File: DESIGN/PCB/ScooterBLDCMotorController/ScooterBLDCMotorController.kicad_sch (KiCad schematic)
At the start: 34 parts, among them J1 M1 OUTPUT, J10 RC_ENABLE, J11 TO M2 ENCODER, J12 M2 INPUT, J13 Conn_01x01_Male, J14 Conn_01x01_Male, J2 TO M1 ENCODER, J3 M1 INPUT, J4 M2 OUTPUT, J5 I2C, J6 TEST SWITCH, J7 RC CH 1, J8 RC CH 2, J9 RC_PWR, U1 , U10 , U2 SN74HC14NR, U3 , U4 Teensy4.0, U5 SN74HC14NR, U6 , U7 , U8 5V_StepUpDown_Voltage_Regulat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, U9 3V_StepUpDown_Voltage_Regulat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

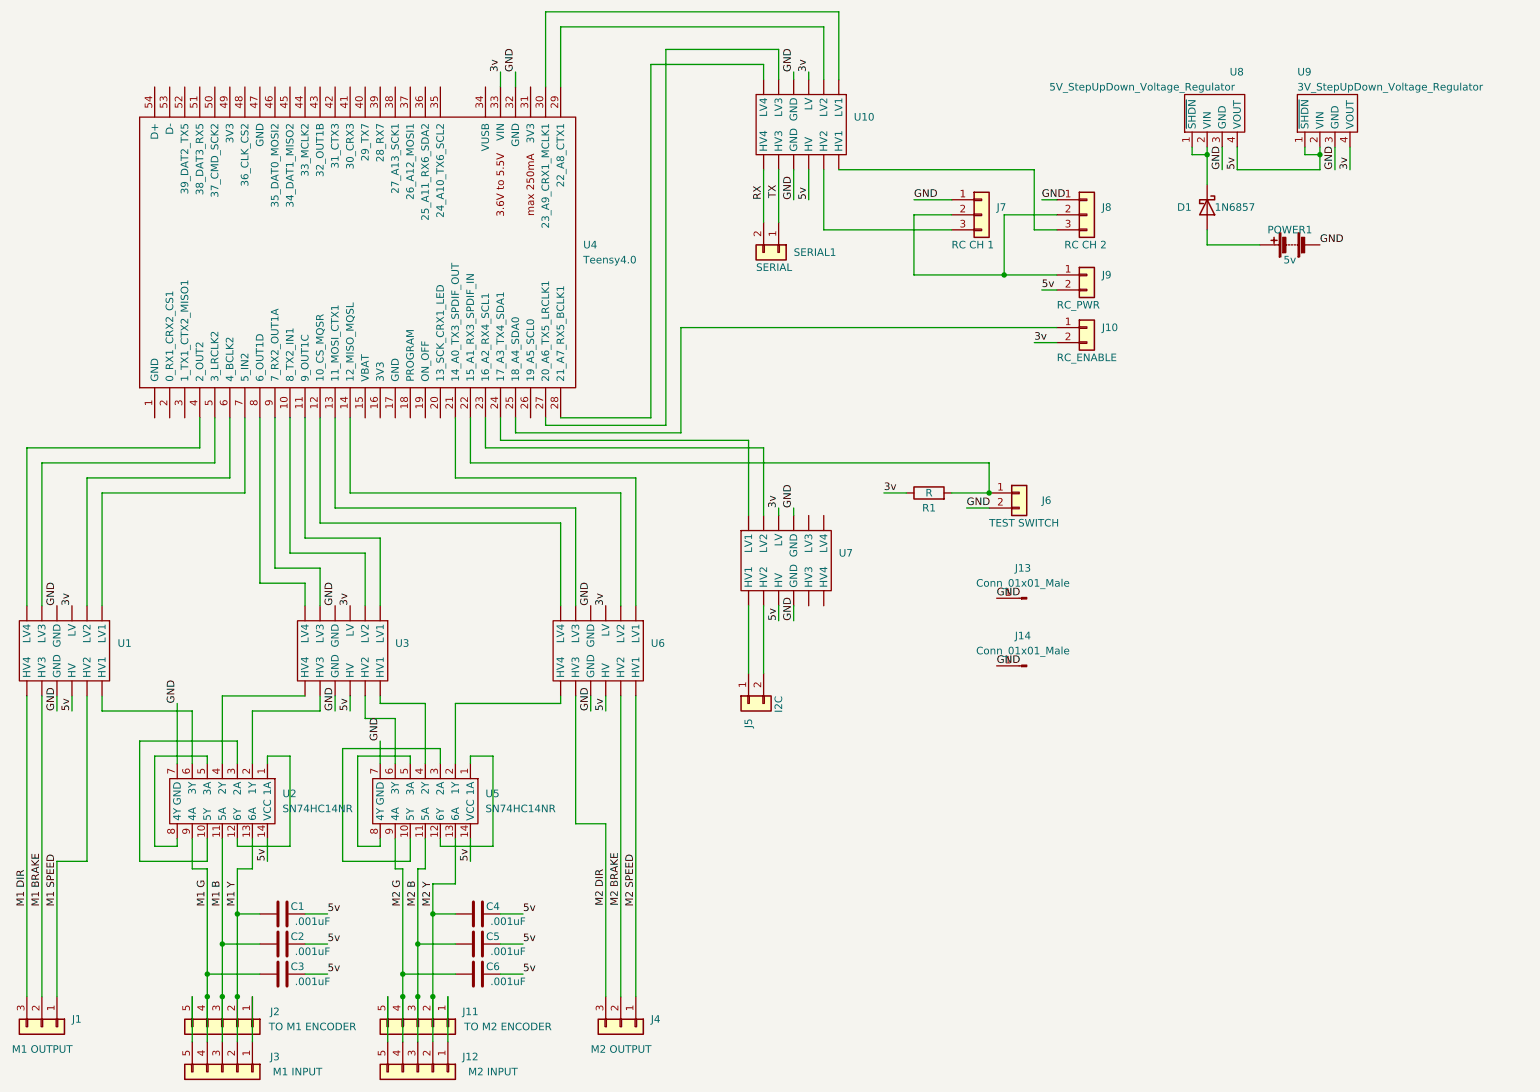
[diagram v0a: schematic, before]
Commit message: Revision 1.3 for PCB
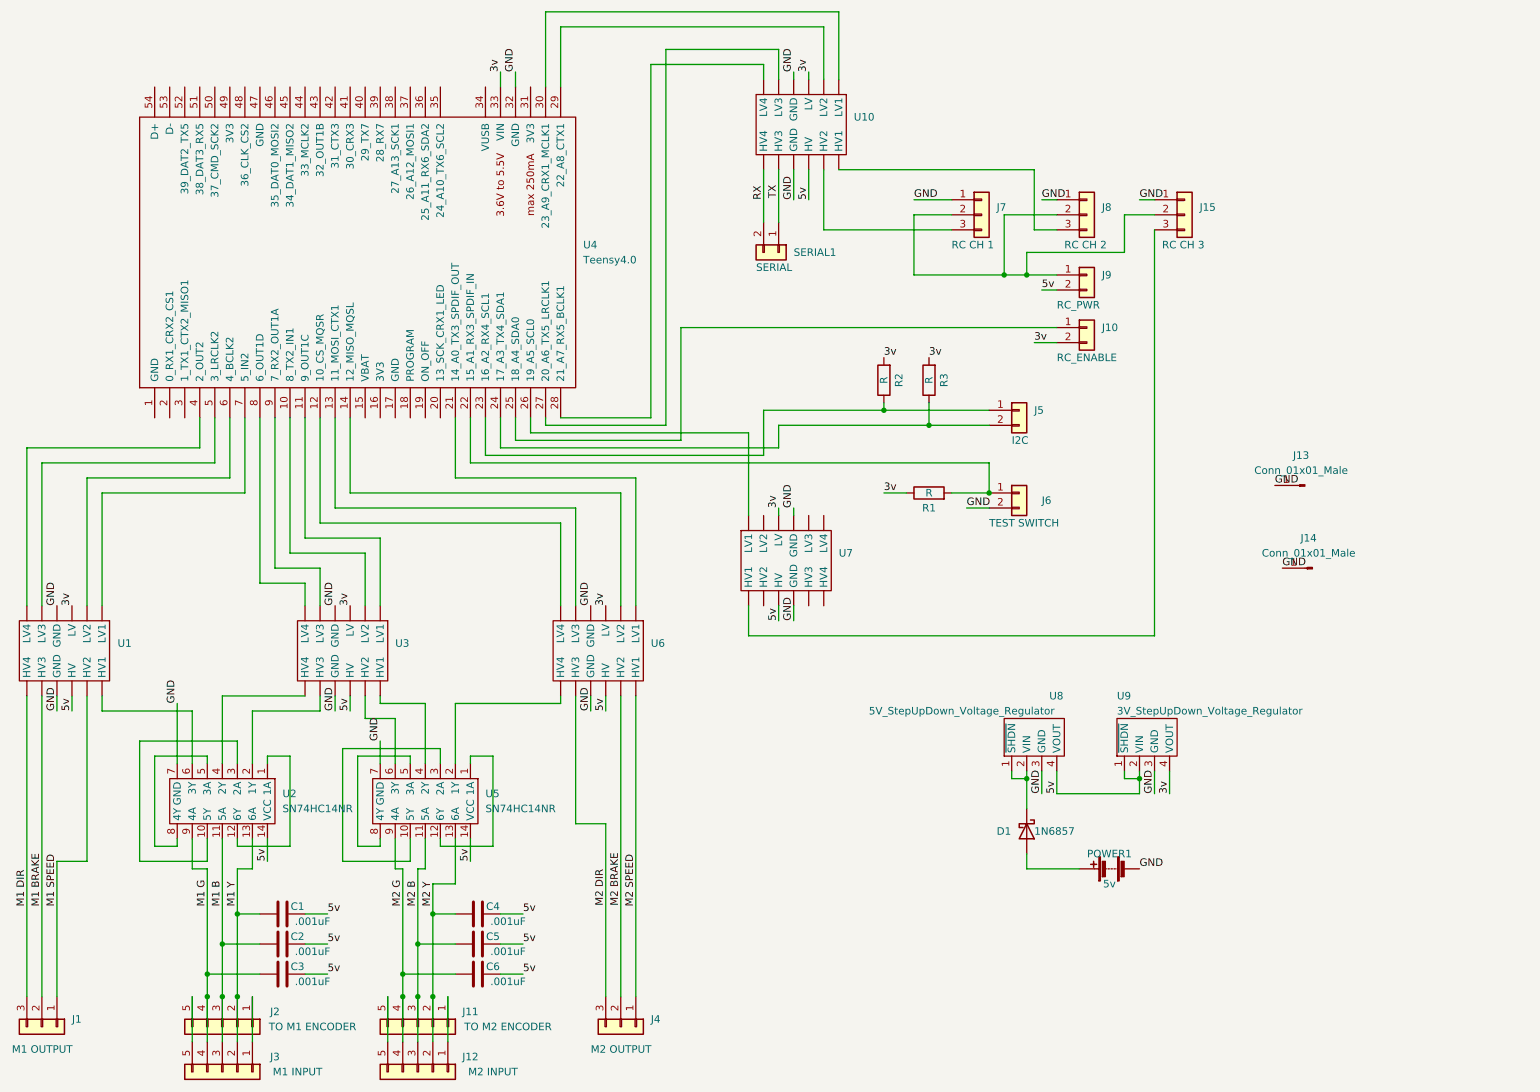
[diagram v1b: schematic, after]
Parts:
- added J15: RC CH 3, Connector_JST:JST_XH_B3B-XH-A_1x03_P2.50mm_Vertical, symbol Connector_Generic:Conn_01x03
- added R2, R3: R, Resistor_THT:R_Axial_DIN0204_L3.6mm_D1.6mm_P7.62mm_Horizontal, symbol Device:R
- C1, C2, C3, C4, C5, C6, D1, J13, J14, R1, U1, U10, U3, U4, U6, U7, U8, U9: now left out of the parts list
- J1, J4: LCSC (none) -> C8393
- J10, J9: LCSC (none) -> C5116481
- J11, J2: LCSC (none) -> C157991
- J12, J3: LCSC (none) -> C395854
- J5, J6, POWER1, SERIAL1: LCSC (none) -> C158012
- J7, J8: LCSC (none) -> C161870
- U2, U5: LCSC (none) -> C2907
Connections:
- net 3v: now also R2.2, R3.2
- net GND: now also J15.1 (Pin_1)
- net at J7.2 (Pin_2), J8.2 (Pin_2), J9.1 (Pin_1): now also J15.2 (Pin_2)
- net at J5.1 (Pin_1): now also U4.23 (16_A2_RX4_SCL1), R2.1; no longer U7.6 (HV1)
- net at J5.2 (Pin_2): now also U4.24 (17_A3_TX4_SDA1), R3.1; no longer U7.5 (HV2)
- net at U7.8 (LV2): no longer U4.23 (16_A2_RX4_SCL1)
- net at U7.7 (LV1): now also U4.26 (19_A5_SCL0); no longer U4.24 (17_A3_TX4_SDA1)
- new net: J15.3 (Pin_3), U7.6 (HV1)
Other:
- moved on the sheet: D1, J13, J14, J5, POWER1, U8, U9
